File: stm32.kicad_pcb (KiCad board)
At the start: 2 copper layers, 49 parts, among them IC1 LTC3621EMS8E-3.3#PBF, J1 TC2030, J2 USB_C_Receptacle_PowerOnly_6P, SW1 SW_Push, U1 STM32F411CEUx, U2 BMI088, U3 BMP388, U4 W25Q128JVSIQ, U5 TP4056-42-ESOP8, U6 AP63203WU, Y1 Crystal_GND24

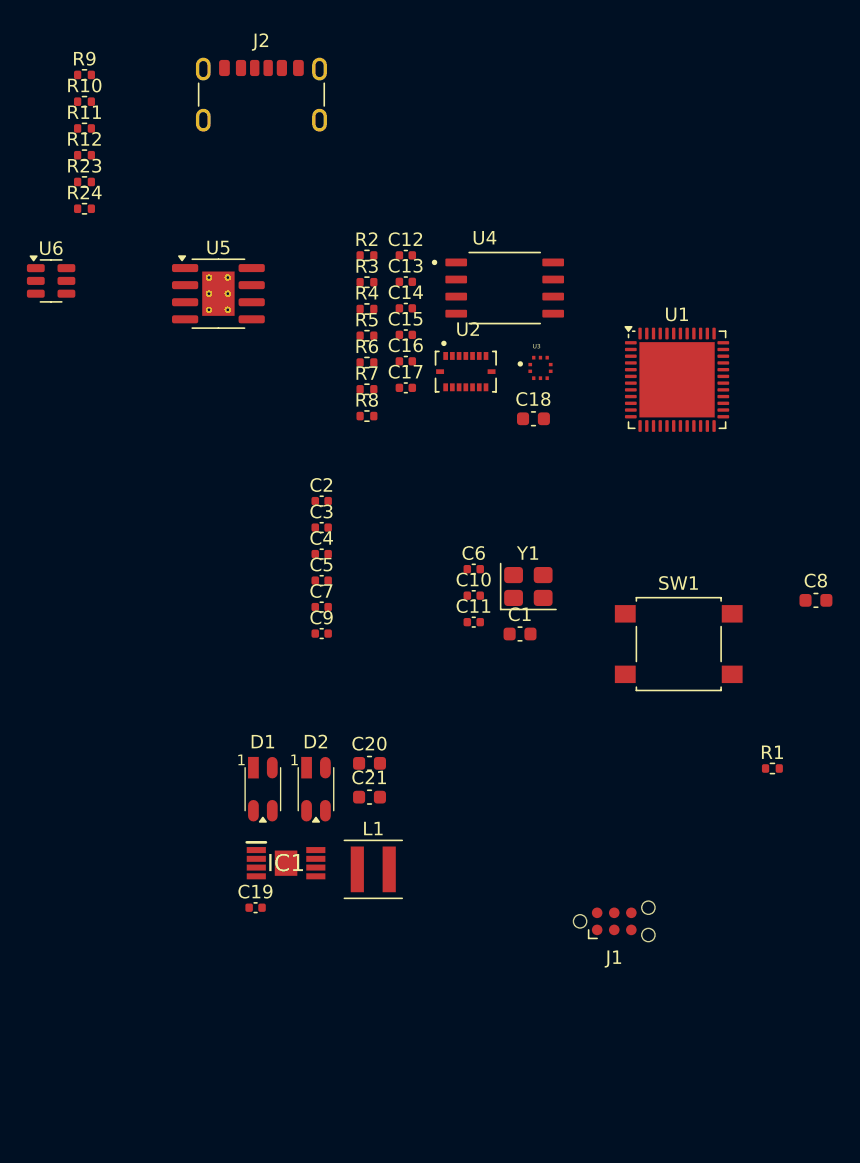
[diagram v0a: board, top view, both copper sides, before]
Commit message: next steps
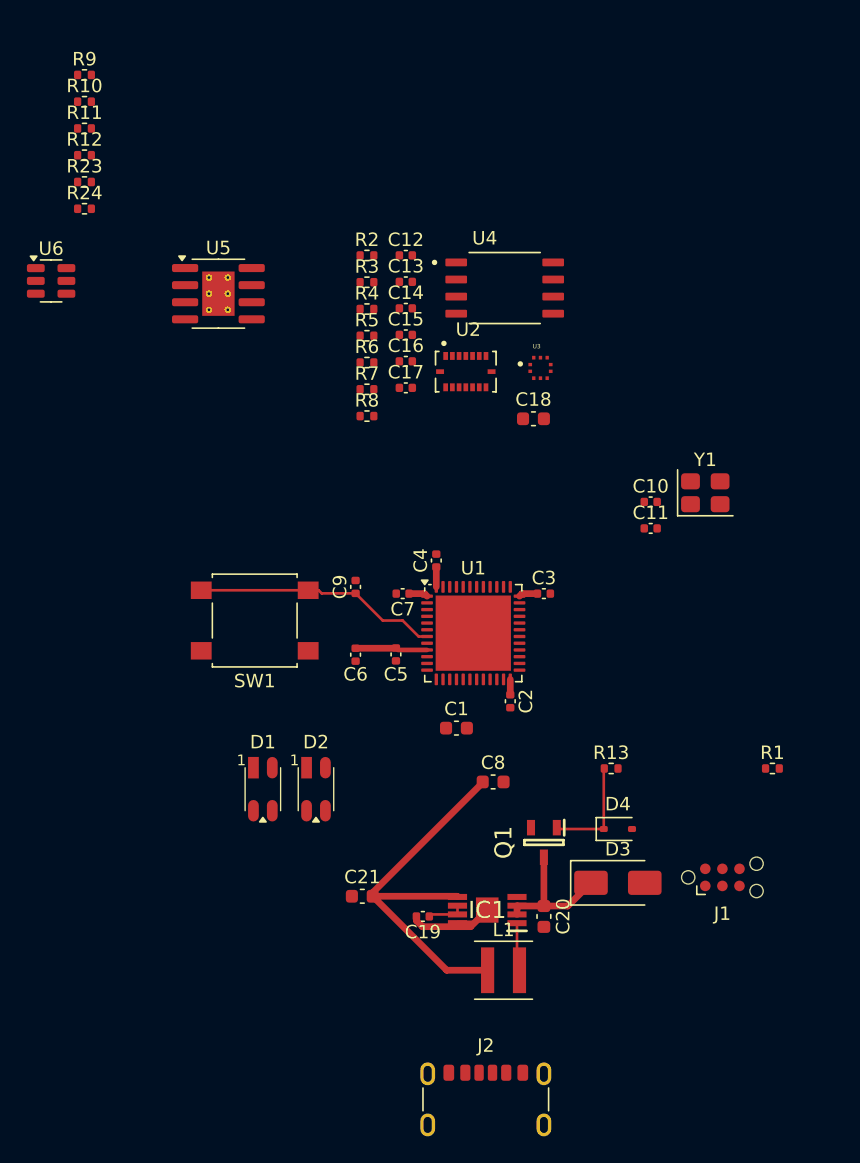
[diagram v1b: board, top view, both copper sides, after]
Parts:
- added D3: SS14, Diode_SMD:D_SMA, F.Cu at (147.5, 92.5)
- added D4: 1N4148WS, Diode_SMD:D_SOD-323, F.Cu at (147.5, 88.5)
- added Q1: DMG2305UX, Custom_Library:DMG2305UX, F.Cu at (142.0, 89.5)
- added R13: 100k, Resistor_SMD:R_0402_1005Metric, F.Cu at (147.0, 84.0)
- Y1: value Crystal_GND24 -> 25MHz
- moved J2 76.5 mm to (137.7, 109.7)
- moved SW1 31.6 mm to (120.5, 73.0), turned to 180 degrees
- moved C8 27.5 mm to (138.2, 85.0)
- moved U1 24.2 mm to (136.8, 73.9)
- moved C2 20.4 mm to (139.5, 79.0), turned to -90 degrees
- moved C20 17.3 mm to (142.0, 95.0), turned to -90 degrees
- moved C3 17.2 mm to (142.0, 71.0)
- moved IC1 15.4 mm to (137.8, 94.5), turned to 180 degrees
- moved C10 14.9 mm to (149.9, 64.2)
- moved C11 14.9 mm to (149.9, 66.2)
- moved Y1 14.9 mm to (154.0, 63.5)
- moved C19 12.5 mm to (133.0, 95.0), turned to 180 degrees
- moved L1 12.2 mm to (139.0, 99.0)
- moved C6 10.8 mm to (128.0, 75.5), turned to -90 degrees
- moved J1 8.68 mm to (155.3, 92.1)
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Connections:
- net +5V renamed /VBUS_5V
- C19 pad 1: GND -> Net-(IC1-INTVCC)
- C19 pad 2: Net-(IC1-INTVCC) -> GND
- IC1 pad 7: unconnected-(IC1-MODE/SYNC-Pad7) -> Net-(IC1-INTVCC)
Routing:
- net +3.3V: track 0.00 -> 39.6 mm
- net /NRST: track 0.00 -> 18.3 mm
- net /VIN_BUCK: track 0.00 -> 10.5 mm
- net GND: track 0.00 -> 8.89 mm
- net /GATE_LS: track 0.00 -> 8.05 mm
- net Net-(IC1-SW): track 0.00 -> 3.58 mm
- net Net-(IC1-INTVCC): track 0.00 -> 2.91 mm
